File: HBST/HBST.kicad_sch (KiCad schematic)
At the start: 38 parts, among them J1 Conn_01x06_Pin, J2 Conn_01x02, J3 Conn_01x04_Pin, J4 Conn_01x13_Pin, J5 Conn_01x09_Pin, J6 Conn_01x02, J7 Conn_01x02, J8 Conn_01x02

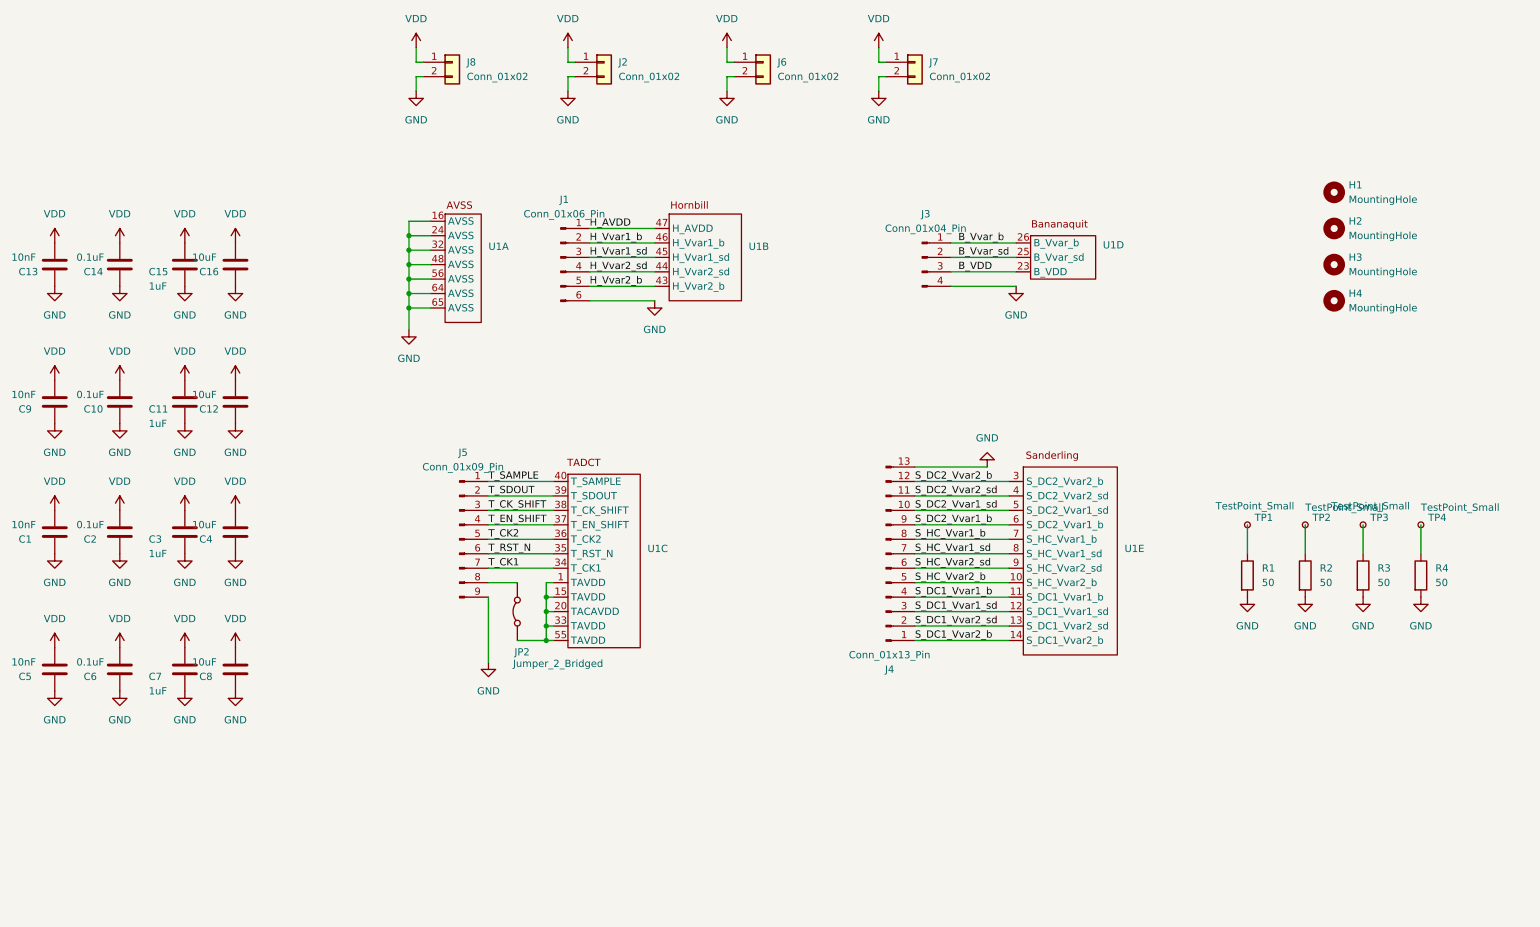
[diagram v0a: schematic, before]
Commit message: minor update
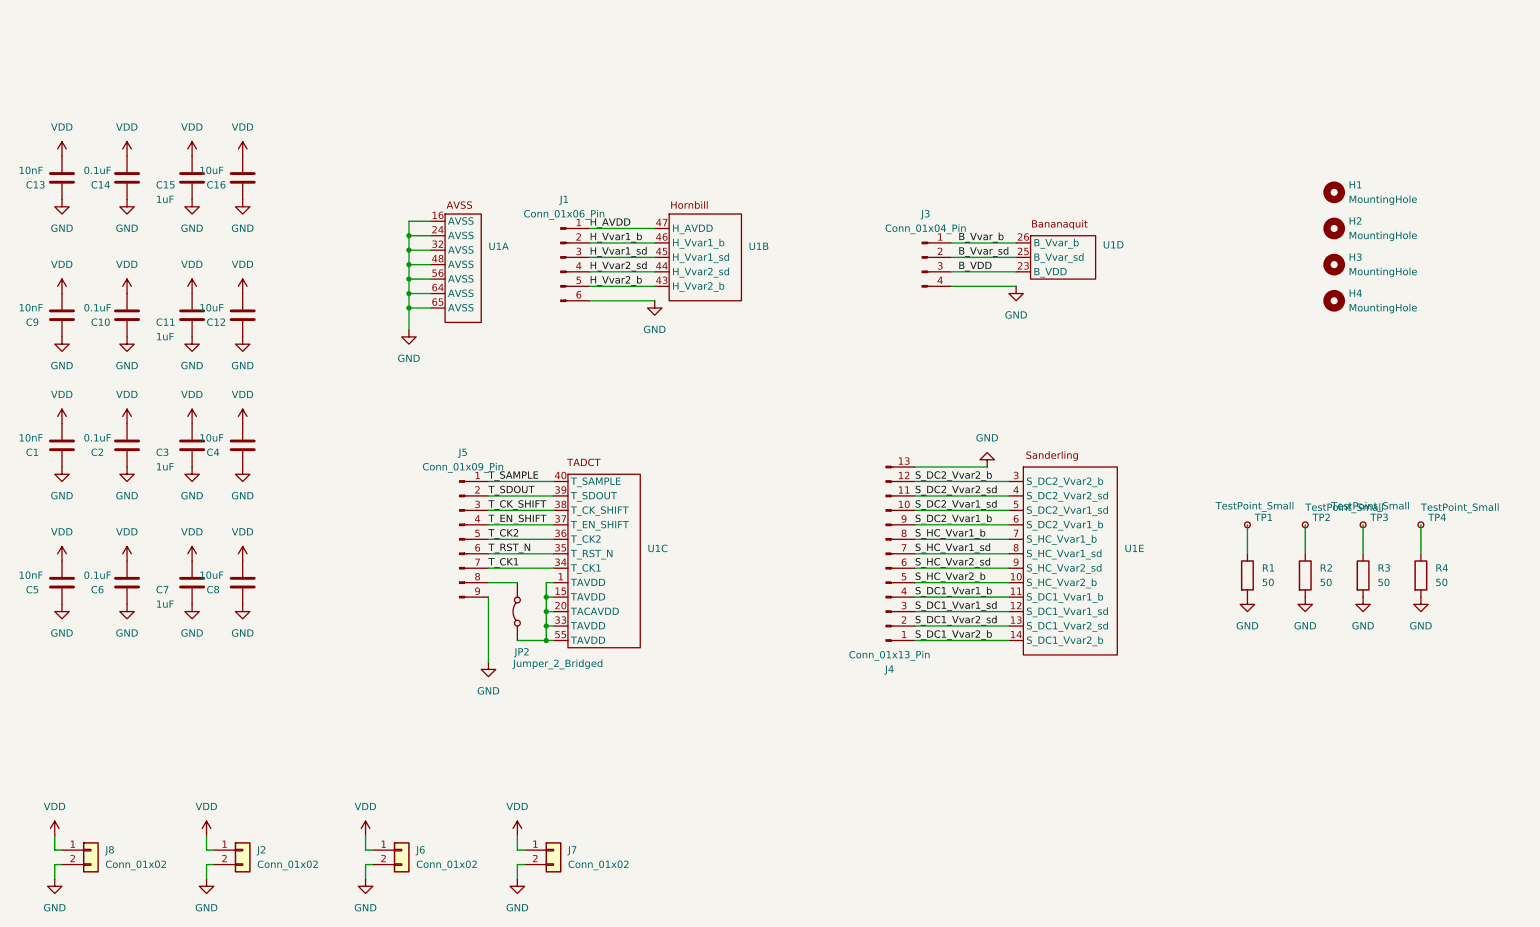
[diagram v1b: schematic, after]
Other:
- moved on the sheet: C1, C10, C11, C12, C13, C14, C15, C16, C2, C3, C4, C5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
